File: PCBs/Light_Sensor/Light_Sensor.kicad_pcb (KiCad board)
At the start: 2 copper layers, 10.2 x 30.5 mm, 5 parts, among them J2 Conn_01x03

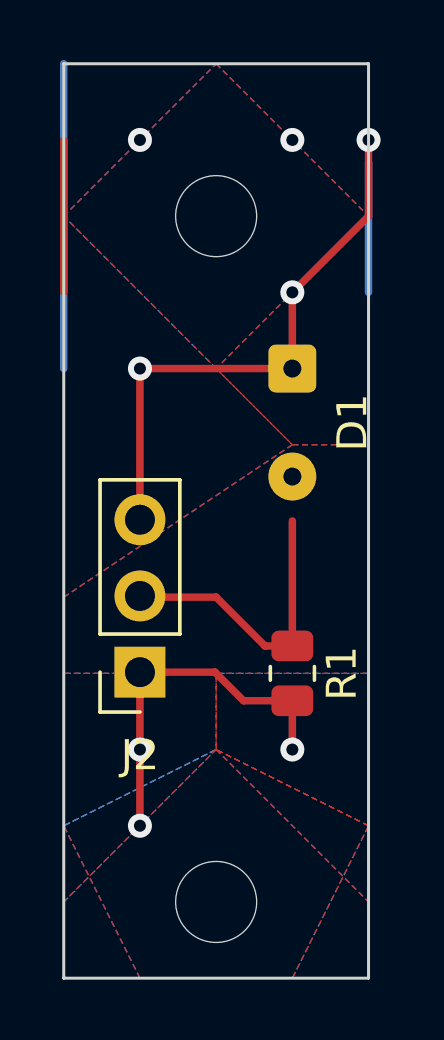
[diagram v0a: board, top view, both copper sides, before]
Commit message: fixed trace
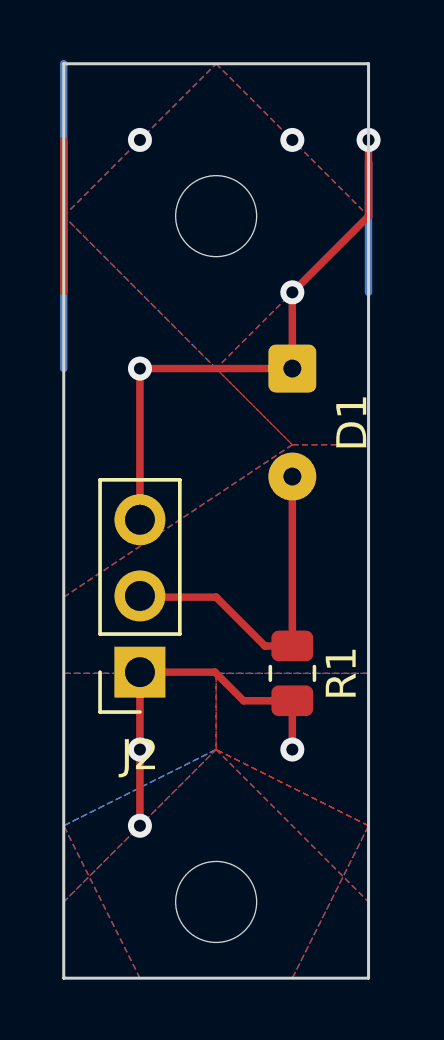
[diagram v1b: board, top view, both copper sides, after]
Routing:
- net Net-(D1-A): track 9.92 -> 11.4 mm
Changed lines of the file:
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@@
   (segment (start 142.24 71.12) (end 142.24 76.2) (width 0.25) (layer "F.Cu") (net 0))
   (segment (start 152.4 76.2) (end 152.4 71.845) (width 0.25) (layer "B.Cu") (net 0))
-  (segment (start 149.86 83.82) (end 149.86 87.9875) (width 0.25) (layer "F.Cu") (net 1))
+  (segment (start 149.86 82.34) (end 149.86 87.9875) (width 0.25) (layer "F.Cu") (net 1))
   (segment (start 149.86 87.9875) (end 148.9475 87.9875) (width 0.25) (layer "F.Cu") (net 1))
   (segment (start 147.32 86.36) (end 144.78 86.36) (width 0.25) (layer "F.Cu") (net 1))
